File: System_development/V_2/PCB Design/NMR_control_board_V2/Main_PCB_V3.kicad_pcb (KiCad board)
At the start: 2 copper layers, 35.1 x 57.4 mm, 18 parts

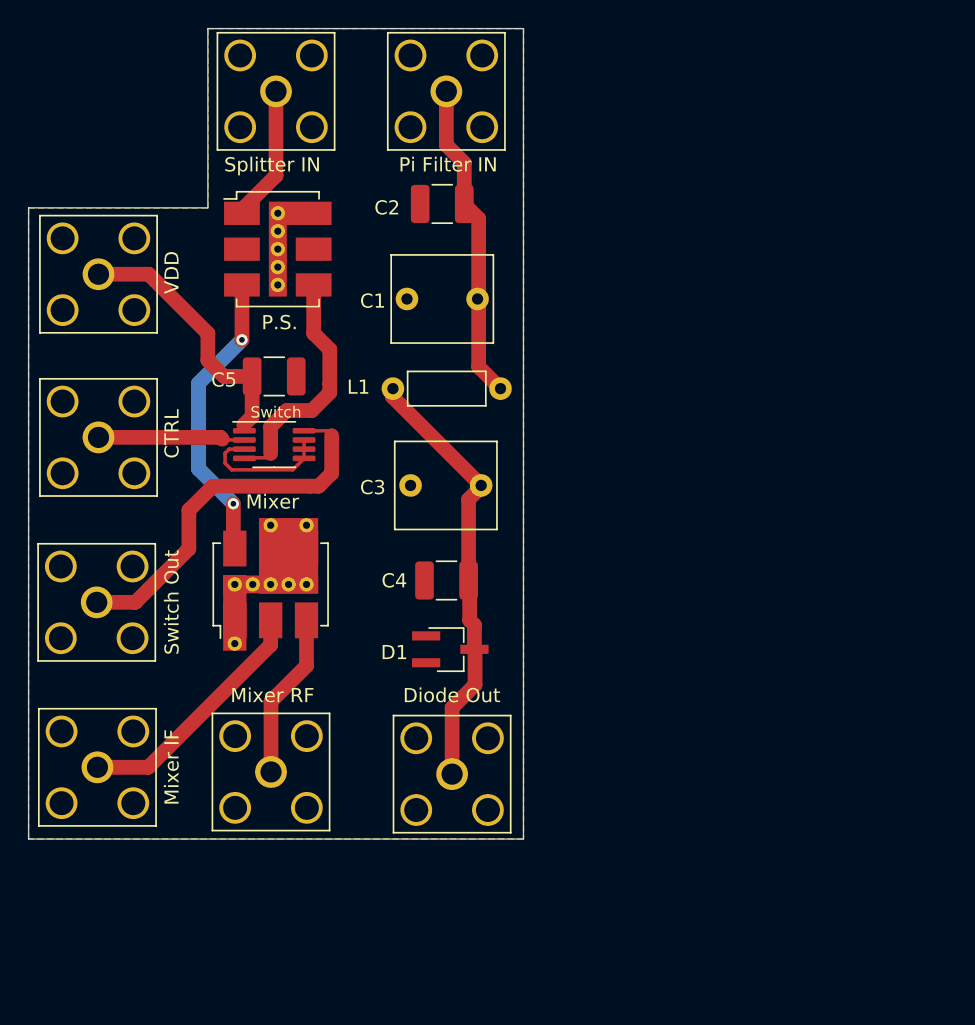
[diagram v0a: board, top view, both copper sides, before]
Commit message: General updates
PCBs & Matlab processing edits
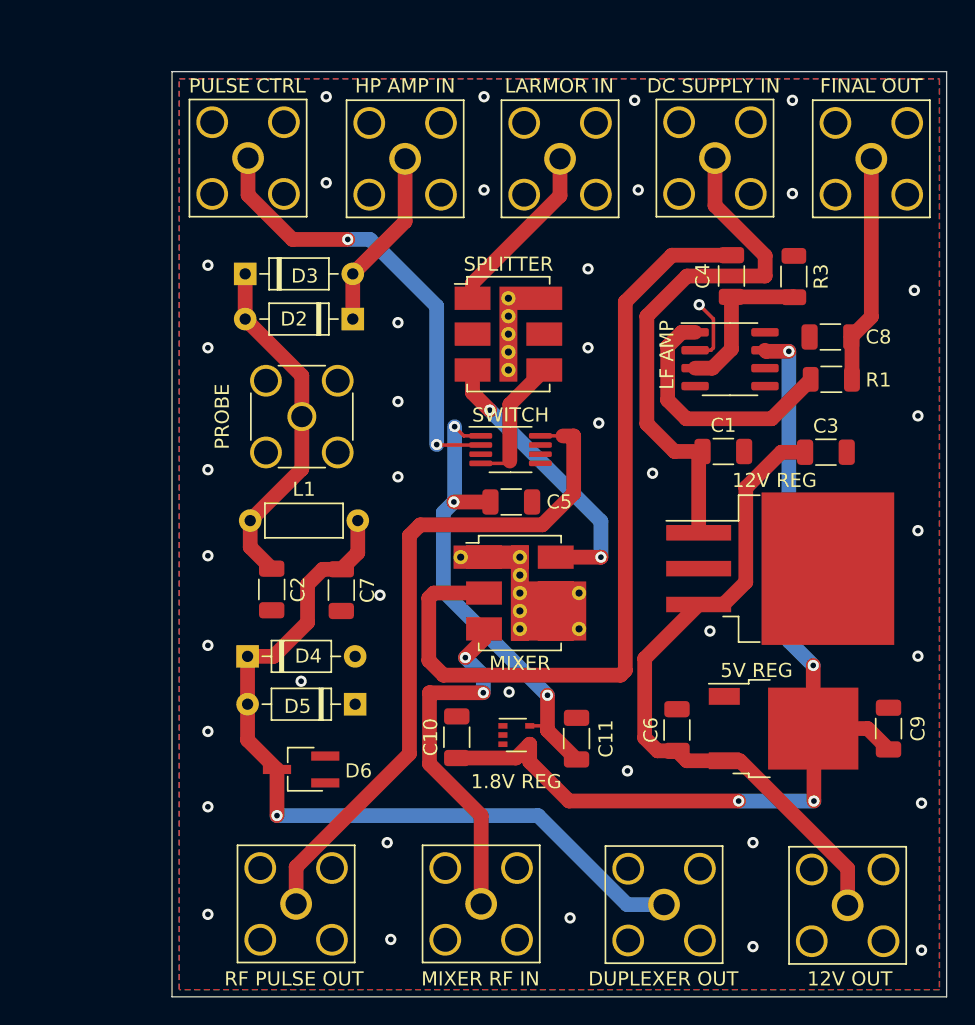
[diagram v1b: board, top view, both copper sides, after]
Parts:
- removed CTRL, VDD: Conn_Coaxial, Connector_Coaxial:SMA_Amphenol_132203-12_Horizontal
- removed D1: D_Schottky_x2_Serial_AKC, Package_TO_SOT_SMD:TSOT-23_HandSoldering
- removed Diode Out: Conn_Coaxial, Connector_Coaxial:SMA_Amphenol_132203-12_Horizontal
- removed Mixer: ADE-6, RF_Mini-Circuits:Mini-Circuits_CD542_LandPatternPL-052
- removed Mixer IF: Conn_Coaxial, Connector_Coaxial:SMA_Amphenol_132203-12_Horizontal
- removed Mixer RF: Conn_Coaxial, Connector_Coaxial:SMA_Amphenol_132203-12_Horizontal
- removed P.S.: ADP-2-1W, RF_Mini-Circuits:Mini-Circuits_CD636_LandPatternPL-035
- removed Pi Filter IN: Conn_Coaxial, Connector_Coaxial:SMA_Amphenol_132203-12_Horizontal
- removed Splitter IN: Conn_Coaxial, Connector_Coaxial:SMA_Amphenol_132203-12_Horizontal
- removed Switch: ADG901BRMZ, Package_SO:MSOP-8_3x3mm_P0.65mm
- removed Switch Out: Conn_Coaxial, Connector_Coaxial:SMA_Amphenol_132203-12_Horizontal
- added 1.8V REG: NCP715-1.8V, Package_TO_SOT_SMD:SOT-353_SC-70-5, F.Cu at (118.4, 113.5)
- added 12V OUT: Conn_Coaxial, Connector_Coaxial:SMA_Amphenol_132203-12_Horizontal, F.Cu at (141.8, 125.6)
- added 12V REG: LM7812_TO220, Package_TO_SOT_SMD:TO-263-3_TabPin2, F.Cu at (137.1, 101.8)
- added 5V REG: NCP1117-5.0_TO252, Package_TO_SOT_SMD:TO-252-2, F.Cu at (137.3, 113.1)
- added C10: 1 uF, Capacitor_SMD:C_1206_3216Metric, F.Cu at (114.1, 113.7)
- added C11: 1 uF, Capacitor_SMD:C_1206_3216Metric, F.Cu at (122.6, 113.8)
- added C6: 10 uF, Capacitor_SMD:C_1206_3216Metric, F.Cu at (129.7, 113.2)
- added C7: C, Capacitor_SMD:C_1206_3216Metric, F.Cu at (106.0, 103.3)
- added C8: C, Capacitor_SMD:C_1206_3216Metric, F.Cu at (140.6, 85.3)
- added C9: 10 uF, Capacitor_SMD:C_1206_3216Metric, F.Cu at (144.7, 113.1)
- added D2: 1N4148, Diode_THT:D_DO-35_SOD27_P7.62mm_Horizontal, F.Cu at (106.8, 84.1)
- added D3: 1N4148, Diode_THT:D_DO-35_SOD27_P7.62mm_Horizontal, F.Cu at (99.2, 80.9)
- added D4: 1N4148, Diode_THT:D_DO-35_SOD27_P7.62mm_Horizontal, F.Cu at (99.3, 108.0)
- added D5: 1N4148, Diode_THT:D_DO-35_SOD27_P7.62mm_Horizontal, F.Cu at (107.0, 111.4)
- added D6: D_Schottky_Dual_Series_AKC, Package_TO_SOT_SMD:TSOT-23_HandSoldering, F.Cu at (103.1, 116.0)
- added DC SUPPLY IN: Conn_Coaxial, Connector_Coaxial:SMA_Amphenol_132203-12_Horizontal, F.Cu at (132.4, 72.7)
- added DUPLEXER OUT: Conn_Coaxial, Connector_Coaxial:SMA_Amphenol_132203-12_Horizontal, F.Cu at (128.8, 125.5)
- added FINAL OUT: Conn_Coaxial, Connector_Coaxial:SMA_Amphenol_132203-12_Horizontal, F.Cu at (143.5, 72.7)
- added HP AMP IN: Conn_Coaxial, Connector_Coaxial:SMA_Amphenol_132203-12_Horizontal, F.Cu at (110.5, 72.7)
- added LARMOR IN: Conn_Coaxial, Connector_Coaxial:SMA_Amphenol_132203-12_Horizontal, F.Cu at (121.5, 72.7)
- added LF AMP: MAX4462 (8-SOIC), Package_SO:SOIC-8_3.9x4.9mm_P1.27mm, F.Cu at (133.5, 86.9)
- added MIXER: ADE-6, RF_Mini-Circuits:Mini-Circuits_CD542_LandPatternPL-052, F.Cu at (118.6, 103.5)
- added MIXER RF IN: Conn_Coaxial, Connector_Coaxial:SMA_Amphenol_132203-12_Horizontal, F.Cu at (115.9, 125.5)
- added PROBE: Conn_Coaxial, Connector_Coaxial:SMA_Amphenol_132291-12_Vertical, F.Cu at (103.2, 91.0)
- added PULSE CTRL: Conn_Coaxial, Connector_Coaxial:SMA_Amphenol_132203-12_Horizontal, F.Cu at (99.4, 72.7)
- added R1: R, Resistor_SMD:R_1206_3216Metric, F.Cu at (140.7, 88.3)
- added R3: R, Resistor_SMD:R_1206_3216Metric, F.Cu at (138.0, 81.1)
- added RF PULSE OUT: Conn_Coaxial, Connector_Coaxial:SMA_Amphenol_132203-12_Horizontal, F.Cu at (102.8, 125.5)
- added SPLITTER: ADP-2-1W, RF_Mini-Circuits:Mini-Circuits_CD636_LandPatternPL-035, F.Cu at (117.8, 85.1)
- added SWITCH: ADG901BRMZ, Package_SO:MSOP-8_3x3mm_P0.65mm, F.Cu at (118.0, 93.3)
- C1: value CTRIM -> 0.33 uF; footprint Capacitor_THT:C_Rect_L7.0mm_W6.0mm_P5.00mm -> Capacitor_SMD:C_1206_3216Metric
- C2, C4: footprint Capacitor_SMD:C_1210_3225Metric_Pad1.33x2.70mm_HandSolder -> Capacitor_SMD:C_1206_3216Metric
- C3: value CTRIM -> 1 uF; footprint Capacitor_THT:C_Rect_L7.0mm_W6.0mm_P5.00mm -> Capacitor_SMD:C_1206_3216Metric
- C5: value C -> 0.1 uF; footprint Capacitor_SMD:C_1210_3225Metric_Pad1.33x2.70mm_HandSolder -> Capacitor_SMD:C_1206_3216Metric
- moved C2 29.9 mm to (101.0, 103.2), turned to -90 degrees
- moved C4 29.5 mm to (133.6, 81.0), turned to -90 degrees
- moved C3 24.5 mm to (140.3, 93.5), turned to 0 degrees
- moved C1 20.5 mm to (133.0, 93.5), turned to 0 degrees
- moved L1 20.0 mm to (99.5, 98.3), turned to 0 degrees
- moved C5 19.0 mm to (118.0, 97.0), turned to 180 degrees
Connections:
- C2 pad 1: Net-(C1-Pad1) -> Net-(C2-Pad1)
- C4 pad 1: Net-(C3-Pad1) -> Net-(C4-Pad1)
- C4 pad 2: GND -> Net-(C4-Pad2)
- C5 pad 1: Net-(C5-Pad1) -> GND
- C5 pad 2: GND -> Net-(C11-Pad1)
- L1 pad 1: Net-(C1-Pad1) -> Net-(C2-Pad1)
- L1 pad 2: Net-(C3-Pad1) -> Net-(C7-Pad1)
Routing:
- net Net-(C10-Pad1): track 0.00 -> 68.4 mm, vias 0 -> 4
- net Net-(C4-Pad1): track 0.00 -> 58.0 mm
- net Net-(C7-Pad1): track 0.00 -> 56.9 mm, vias 0 -> 1
- net Net-(C11-Pad1): track 0.00 -> 33.9 mm, vias 0 -> 3
- net Net-(C2-Pad1): track 0.00 -> 24.7 mm
- net Net-(J2-Pad1): track 9.83 -> 32.2 mm, vias 0 -> 2
- net Net-(J6-Pad1): track 26.4 -> 48.7 mm
- net Net-(C5-Pad1): track 18.6 -> 0.00 mm
- net Net-(C3-Pad1): track 29.7 -> 47.8 mm
- net Net-(R1-Pad1): track 0.00 -> 18.0 mm
- net Net-(J5-Pad1): track 17.5 -> 0.00 mm
- net Net-(C8-Pad2): track 0.00 -> 16.2 mm
- net Net-(C1-Pad1): track 22.2 -> 37.6 mm
- net Net-(J3-Pad1): track 11.3 -> 25.9 mm, vias 0 -> 2
- net Net-(D2-Pad1): track 0.00 -> 12.9 mm
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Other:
- board size 35.1 x 57.4 mm -> 54.9 x 65.5 mm
- net class 50 Ohm removed
- net class Default removed
- board text added: "NMR CONTROL V2"
- board text removed: "NMR Control V1"
